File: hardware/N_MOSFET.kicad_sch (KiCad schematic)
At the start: 4 parts, among them Q4 Q_NMOS_DGS

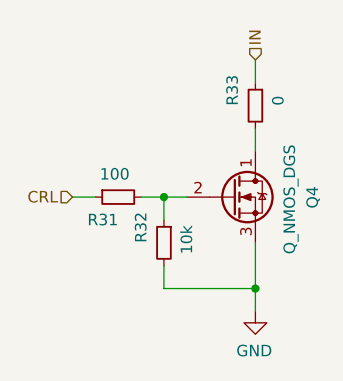
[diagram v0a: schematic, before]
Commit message: fuck
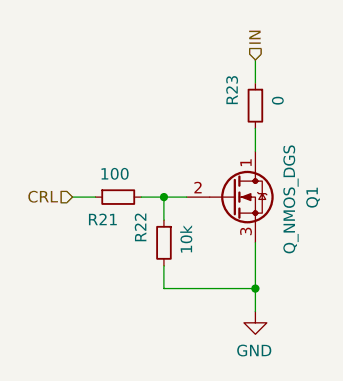
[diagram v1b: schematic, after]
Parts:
- renumbered Q4 to Q1, R31 to R21, R32 to R22, R33 to R23
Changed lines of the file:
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@@
   (symbol (lib_id "Device:Q_NMOS_DGS") (at 161.29 102.87 0)
     (in_bom yes) (on_board yes)
-    (property "Reference" "Q4" (id 0) (at 170.18 104.14 90)
+    (property "Reference" "Q1" (id 0) (at 170.18 104.14 90)
       (effects (font (size 1.27 1.27)) (justify left))
     )
@@
   (symbol (lib_id "Device:R_Small") (at 153.67 107.95 0) (mirror y)
     (in_bom yes) (on_board yes)
-    (property "Reference" "R32" (id 0) (at 151.13 107.95 90)
+    (property "Reference" "R22" (id 0) (at 151.13 107.95 90)
       (effects (font (size 1.27 1.27)) (justify left))
     )
@@
   (symbol (lib_id "Device:R_Small") (at 148.59 102.87 90) (mirror x)
     (in_bom yes) (on_board yes)
-    (property "Reference" "R31" (id 0) (at 148.59 105.41 90)
+    (property "Reference" "R21" (id 0) (at 148.59 105.41 90)
       (effects (font (size 1.27 1.27)) (justify left))
     )
@@
   (symbol (lib_id "Device:R_Small") (at 163.83 92.71 0) (mirror y)
     (in_bom yes) (on_board yes)
-    (property "Reference" "R33" (id 0) (at 161.29 92.71 90)
+    (property "Reference" "R23" (id 0) (at 161.29 92.71 90)
       (effects (font (size 1.27 1.27)) (justify left))
     )
@@
   (symbol (lib_id "power:GND") (at 163.83 115.57 0) (mirror y)
     (in_bom yes) (on_board yes)
-    (property "Reference" "#PWR0125" (id 0) (at 163.83 121.92 0)
+    (property "Reference" "#PWR0106" (id 0) (at 163.83 121.92 0)
       (effects (font (size 1.27 1.27)) hide)
     )
